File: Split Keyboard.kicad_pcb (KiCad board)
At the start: 2 copper layers, 91 parts, among them CN1 1.0-2P WT, CN2 1.0-2P WT, SW1 Switch, SW10 Switch, SW11 Switch, SW12 Switch, SW13 Switch, SW14 Switch, SW15 Switch, SW16 Switch, SW17 Switch, SW18 Switch, SW19 Switch, SW2 Switch, SW20 Switch, SW21 Switch, SW22 Switch, SW23 Switch, SW24 EC11, SW25 Switch, SW26 Switch, SW27 Switch, SW28 Switch, SW29 Switch, SW3 Switch, SW30 Switch, SW31 Switch, SW32 Switch, SW33 Switch, SW34 Switch, SW4 Switch, SW5 Switch, SW6 Switch, SW7 EC11, SW8 Switch, SW9 Switch, U1 XIAO-nRF52840-SMD, U2 XIAO-nRF52840-SMD

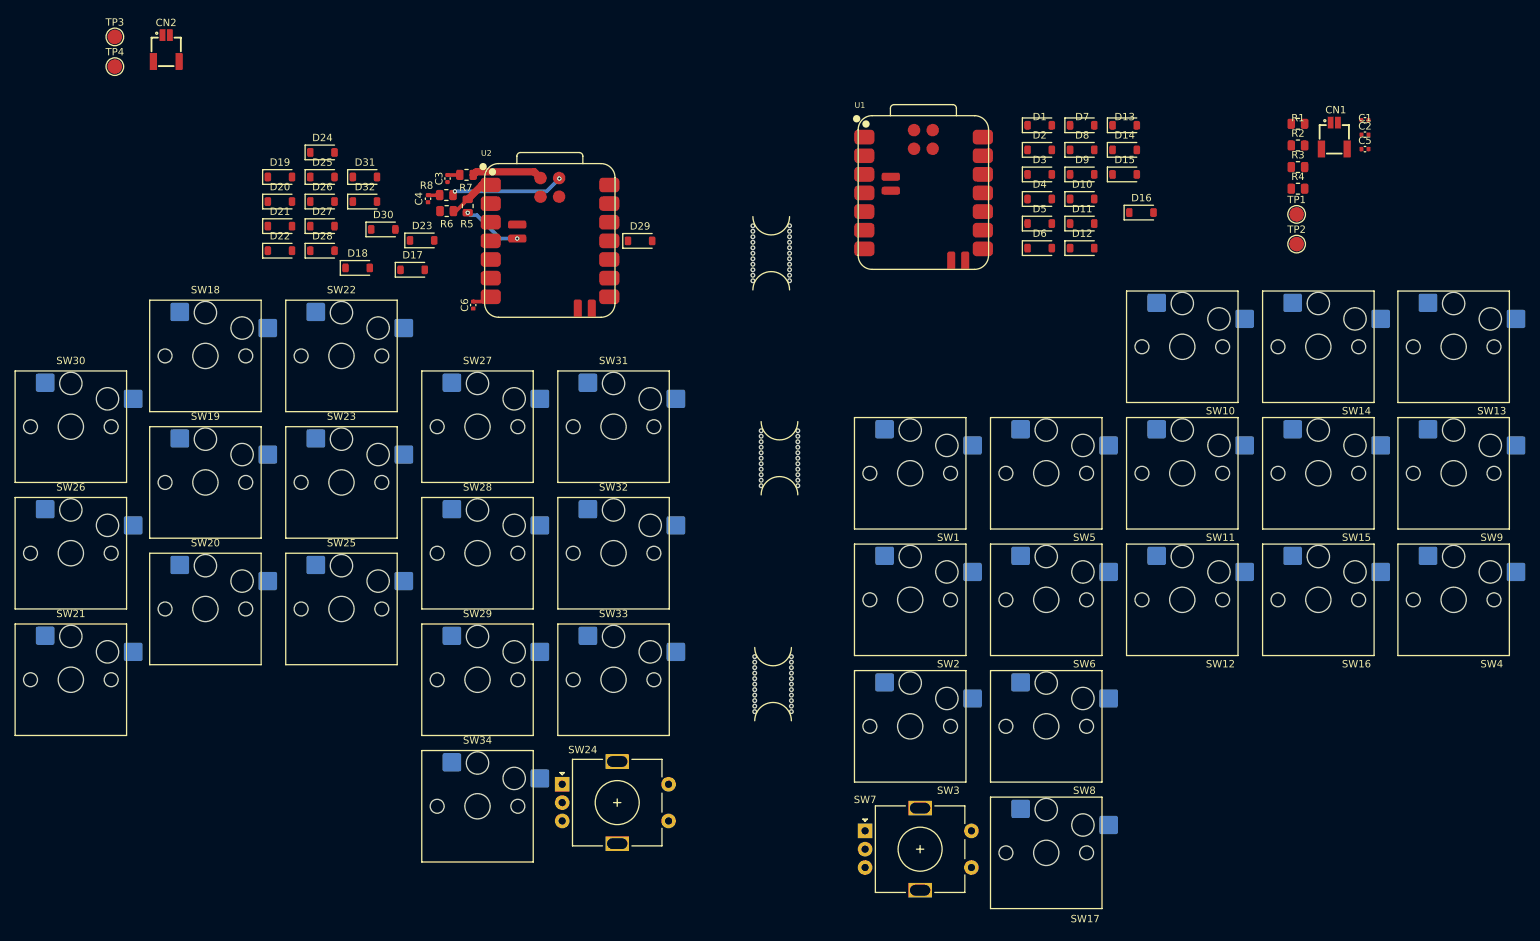
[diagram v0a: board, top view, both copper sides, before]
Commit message: Doing it
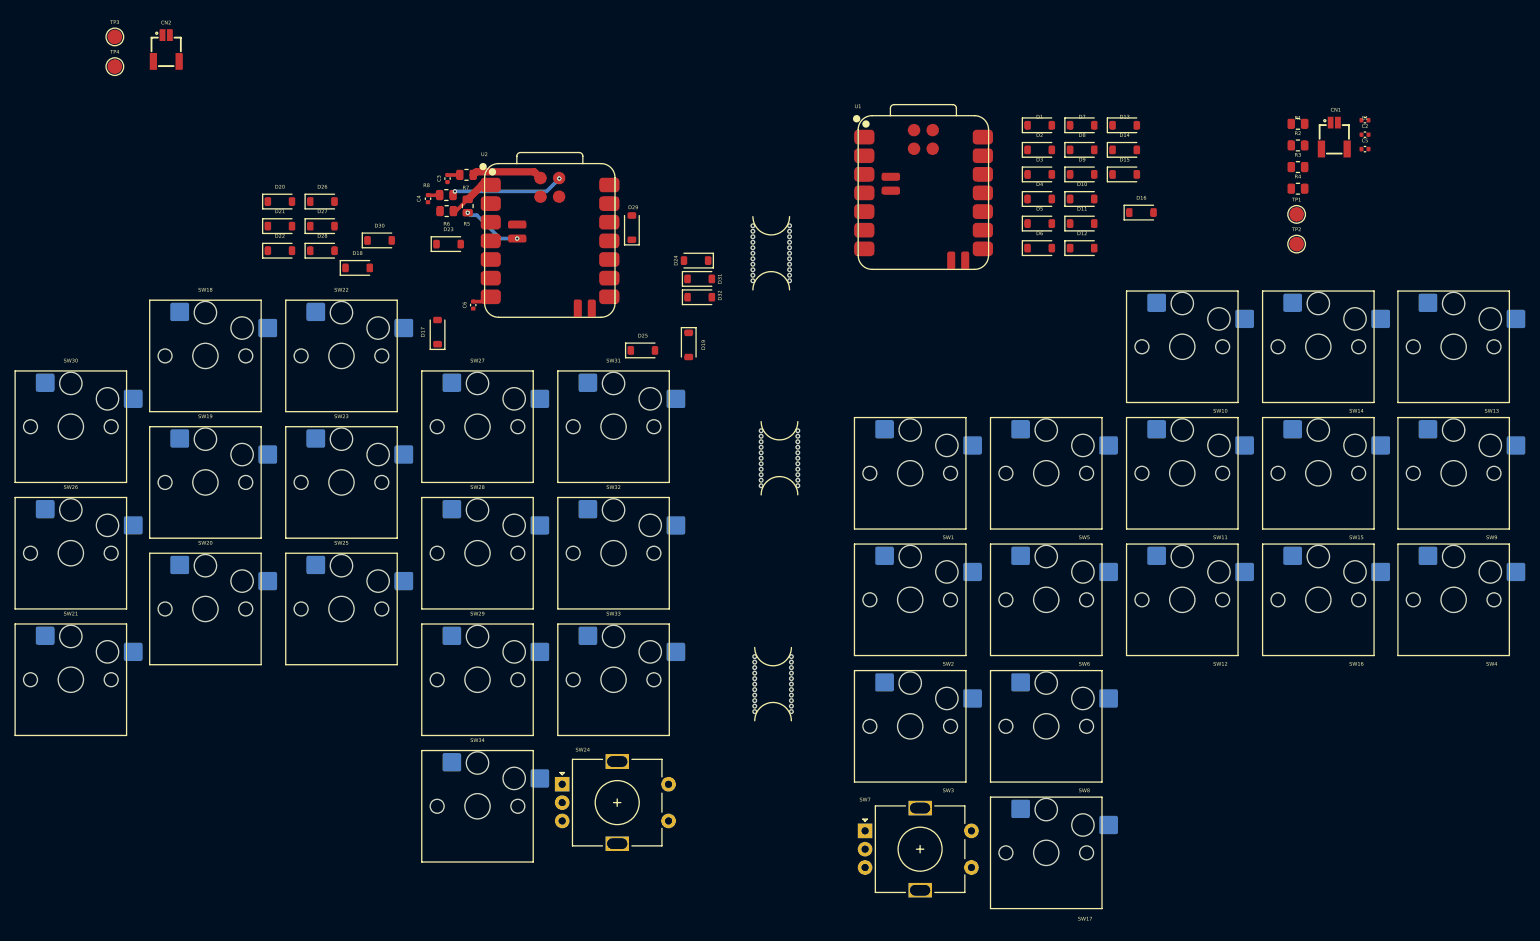
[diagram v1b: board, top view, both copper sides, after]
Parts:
- moved D19 60.3 mm to (154.0, 62.2), turned to -90 degrees
- moved D24 53.0 mm to (155.0, 50.8), turned to 180 degrees
- moved D25 49.7 mm to (147.8, 63.0)
- moved D31 47.7 mm to (155.5, 53.2)
- moved D32 47.5 mm to (155.5, 55.8)
- moved D17 9.15 mm to (119.8, 60.5), turned to 90 degrees
- moved D23 3.63 mm to (121.2, 48.5)
- moved D29 2.13 mm to (146.2, 46.2), turned to 90 degrees
- moved D30 1.58 mm to (111.8, 48.0)
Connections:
- D19 pad 2: /Right/COL1 -> Net-(D19-A)
- D22 pad 2: /Right/COL2 -> Net-(D22-A)
- D3 pad 2: /Left/COL1 -> Net-(D3-A)
- D6 pad 2: /Left/COL2 -> Net-(D6-A)
- SW20 pad 2: /Right/COL1 -> Net-(D19-A)
- SW23 pad 2: /Right/COL2 -> Net-(D22-A)
- SW3 pad 2: /Left/COL1 -> Net-(D3-A)
- SW6 pad 2: /Left/COL2 -> Net-(D6-A)
